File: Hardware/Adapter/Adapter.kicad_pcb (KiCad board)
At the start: 2 copper layers, 52.8 x 32.5 mm, 15 parts, among them J1 GameBoy_LinkPort, Q1 BSS13B, Q2 BSS13B, Q3 BSS13B, Q4 BSS13B, U1 Pico

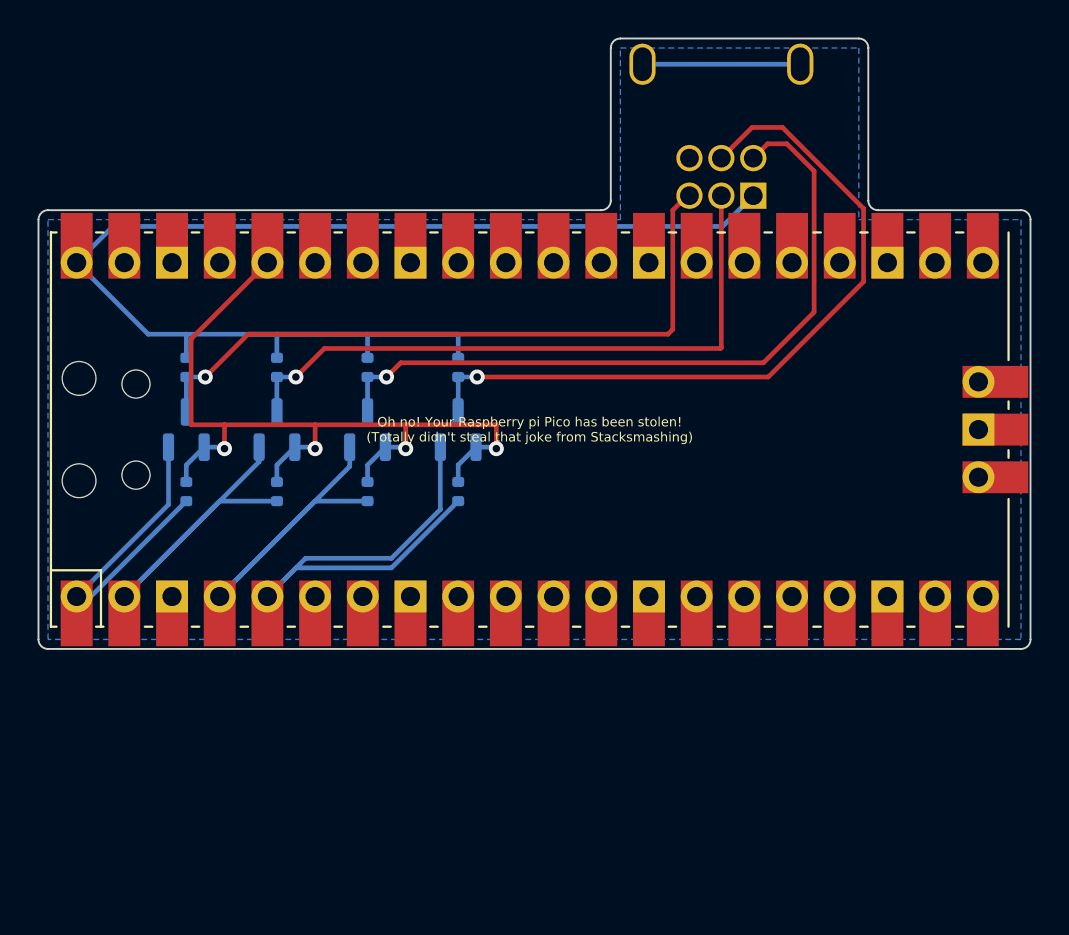
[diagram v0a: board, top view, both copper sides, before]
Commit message: Redid adapter, almost done, but I just wanna code stuff now
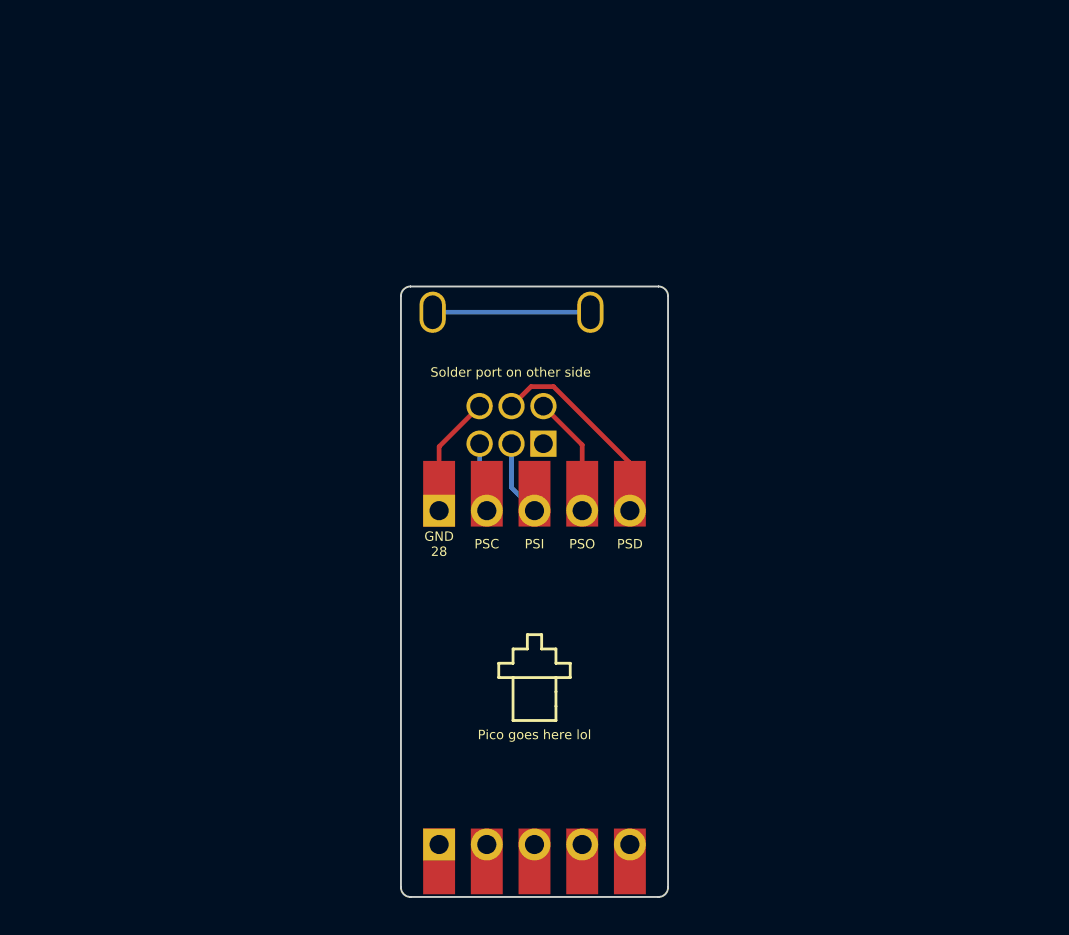
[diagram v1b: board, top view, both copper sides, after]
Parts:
- removed Q1, Q2, Q3, Q4: BSS13B, Package_TO_SOT_SMD:SOT-23
- removed R1, R2, R3, R4, R5, R6, R7, R8: 10k, Resistor_SMD:R_0402_1005Metric
- moved G1 20.9 mm to (152.1, 103.9)
- moved J1 17.3 mm to (152.7, 95.4)
- moved U1 13.2 mm to (152.1, 107.2)
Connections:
- J1 pad 1: +5V -> unconnected-(J1-Pad1)
- J1 pad 2: Net-(J1-Pad2) -> PSO
- J1 pad 3: Net-(J1-Pad3) -> PSI
- J1 pad 4: Net-(J1-Pad4) -> PSD
- J1 pad 5: Net-(J1-Pad5) -> PSC
- U1 pad 13: GND -> unconnected-(U1-Pad13)
- U1 pad 24: unconnected-(U1-Pad24) -> PSD
- U1 pad 25: unconnected-(U1-Pad25) -> PSO
- U1 pad 26: unconnected-(U1-Pad26) -> PSI
- U1 pad 27: unconnected-(U1-Pad27) -> PSC
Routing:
- net +5V: track 64.5 -> 0.00 mm
- net +3V3: track 45.1 -> 0.00 mm, vias 4 -> 0
- net Net-(J1-Pad4): track 39.5 -> 0.00 mm, vias 1 -> 0
- net Net-(J1-Pad2): track 38.7 -> 0.00 mm, vias 1 -> 0
- net Net-(J1-Pad5): track 36.5 -> 0.00 mm, vias 1 -> 0
- net Net-(J1-Pad3): track 34.3 -> 0.00 mm, vias 1 -> 0
- net PSI: track 21.2 -> 4.07 mm
- net PSD: track 26.7 -> 11.0 mm
- net PSO: track 20.8 -> 6.42 mm
- net PSC: track 17.9 -> 3.73 mm
- net GND: track 0.00 -> 6.46 mm
- removed copper zone on B.Cu, net GND
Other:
- board size 52.8 x 32.5 mm -> 14.2 x 32.5 mm
- board text added: "3v3"
- board text added: "GND 28"
- board text added: "PSC"
- board text added: "PSD"
- board text added: "PSI"
- board text added: "PSO"
- board text added: "Pico goes here lol"
- board text added: "Solder port on other side"
- board text added: "TileWorld GBA Thingamabob Made by: Matthew Collier (Squaresweets) Thanks to: DFranx, Nonchip, Lorenzoone, EchelonPrime, Stacksmashing and maciel310 for making this project possible!"
- board text removed: "5v"
- board text removed: "Little bit of extra space for wiring"
- board text removed: "Oh no! Your Raspberry pi Pico has been stolen! (Totally didn't steal that joke from Stacksmashing)"
- board text removed: "TileWorld adapter v.1 Made by: Matthew Collier (Squaresweets) Thanks to: DFranx, Nonchip, Lorenzoone, EchelonPrime, Stacksmashing and maciel310 for making this project possible!"
- board text removed: "level shifter thingamabobs"
